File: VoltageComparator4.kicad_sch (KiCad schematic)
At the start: 6 parts, among them U18 LM324, U19 74LS08

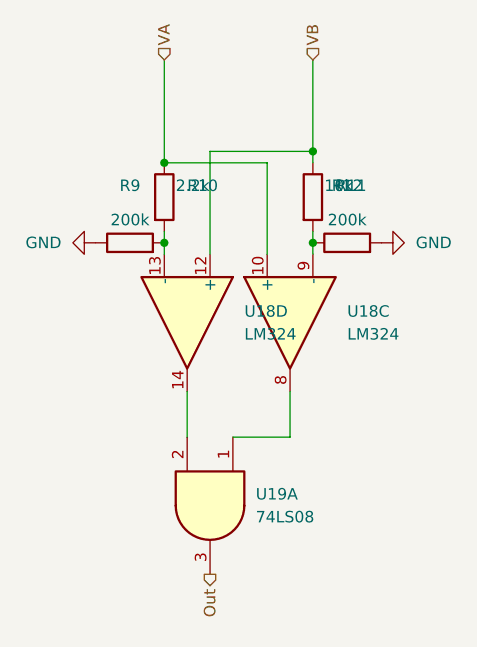
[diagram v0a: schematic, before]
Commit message: Ground and Power Plane?
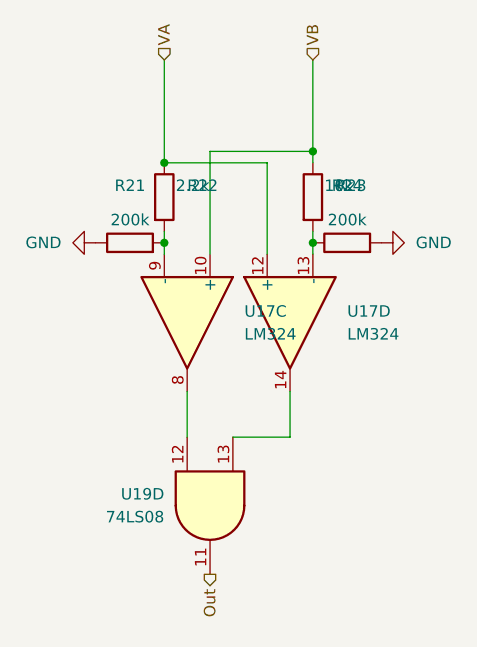
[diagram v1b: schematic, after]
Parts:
- renumbered R9 to R21, R10 to R22, R11 to R23, R12 to R24, U18 to U17
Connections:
- net Out: now also U19.11; no longer U19.3
- net VA: now also U17.12 (+); no longer U17.10 (+)
- net VB: now also U17.10 (+); no longer U17.12 (+)
- net at R21.2, R22.2: now also U17.9 (-); no longer U17.13 (-)
- net at R23.2, R24.1: now also U17.13 (-); no longer U17.9 (-)
- new net: U17.8, U19.12
- new net: U17.14, U19.13
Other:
- moved on the sheet: U19D
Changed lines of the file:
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@@
 	(symbol
 		(lib_id "74xx:74LS08")
-		(at 53.34 96.52 270)
-		(unit 1)
+		(at 53.34 96.52 90)
+		(mirror x)
+		(unit 4)
 		(exclude_from_sim no)
 		(in_bom yes)
@@
 		(dnp no)
 		(property "Reference" "U19"
-			(at 58.42 95.2416 90)
+			(at 48.26 95.2416 90)
 			(effects
 				(font
@@
 		)
 		(property "Value" "74LS08"
-			(at 58.42 97.7816 90)
+			(at 48.26 97.7816 90)
 			(effects
 				(font
@@
 		(dnp no)
 		(fields_autoplaced yes)
-		(property "Reference" "#PWR088"
+		(property "Reference" "#PWR094"
 			(at 78.74 67.31 0)
 			(effects
@@
 		(instances
 			(project "ECE145Mastermind"
-				(path "/8c64fe8a-5d6b-41bc-b3a3-9bda7b2e0f2c/4f59e726-7fd4-4ef0-8dbb-7a41976aa953"
-					(reference "#PWR088")
+				(path "/8c64fe8a-5d6b-41bc-b3a3-9bda7b2e0f2c/d4674d5d-47f2-4c8d-9fae-4e866cda3652"
+					(reference "#PWR094")
 					(unit 1)
 				)
@@
 		(on_board yes)
 		(dnp no)
-		(property "Reference" "R10"
+		(property "Reference" "R22"
 			(at 50.8 60.9599 0)
 			(effects
@@
 		(instances
 			(project "ECE145Mastermind"
-				(path "/8c64fe8a-5d6b-41bc-b3a3-9bda7b2e0f2c/4f59e726-7fd4-4ef0-8dbb-7a41976aa953"
-					(reference "R10")
+				(path "/8c64fe8a-5d6b-41bc-b3a3-9bda7b2e0f2c/d4674d5d-47f2-4c8d-9fae-4e866cda3652"
+					(reference "R22")
 					(unit 1)
 				)
@@
 		(dnp no)
 		(fields_autoplaced yes)
-		(property "Reference" "#PWR087"
+		(property "Reference" "#PWR093"
 			(at 34.29 67.31 0)
 			(effects
@@
 		(instances
 			(project "ECE145Mastermind"
-				(path "/8c64fe8a-5d6b-41bc-b3a3-9bda7b2e0f2c/4f59e726-7fd4-4ef0-8dbb-7a41976aa953"
-					(reference "#PWR087")
+				(path "/8c64fe8a-5d6b-41bc-b3a3-9bda7b2e0f2c/d4674d5d-47f2-4c8d-9fae-4e866cda3652"
+					(reference "#PWR093")
 					(unit 1)
 				)
@@
 		(on_board yes)
 		(dnp no)
-		(property "Reference" "R11"
+		(property "Reference" "R23"
 			(at 67.31 60.9599 0)
 			(effects
@@
 		(instances
 			(project "ECE145Mastermind"
-				(path "/8c64fe8a-5d6b-41bc-b3a3-9bda7b2e0f2c/4f59e726-7fd4-4ef0-8dbb-7a41976aa953"
-					(reference "R11")
+				(path "/8c64fe8a-5d6b-41bc-b3a3-9bda7b2e0f2c/d4674d5d-47f2-4c8d-9fae-4e866cda3652"
+					(reference "R23")
 					(unit 1)
 				)
@@
 		(at 62.23 76.2 90)
 		(mirror x)
-		(unit 3)
+		(unit 4)
 		(exclude_from_sim no)
 		(in_bom yes)
@@
 		(dnp no)
 		(fields_autoplaced yes)
-		(property "Reference" "U18"
+		(property "Reference" "U17"
 			(at 68.58 74.9299 90)
 			(effects
@@
 		(instances
 			(project "ECE145Mastermind"
-				(path "/8c64fe8a-5d6b-41bc-b3a3-9bda7b2e0f2c/4f59e726-7fd4-4ef0-8dbb-7a41976aa953"
-					(reference "U18")
-					(unit 3)
+				(path "/8c64fe8a-5d6b-41bc-b3a3-9bda7b2e0f2c/d4674d5d-47f2-4c8d-9fae-4e866cda3652"
+					(reference "U17")
+					(unit 4)
 				)
 			)
@@
 		(lib_id "Amplifier_Operational:LM324")
 		(at 50.8 76.2 270)
-		(unit 4)
+		(unit 3)
 		(exclude_from_sim no)
 		(in_bom yes)
@@
 		(dnp no)
 		(fields_autoplaced yes)
-		(property "Reference" "U18"
+		(property "Reference" "U17"
 			(at 57.15 74.9299 90)
 			(effects
@@
 		(instances
 			(project "ECE145Mastermind"
-				(path "/8c64fe8a-5d6b-41bc-b3a3-9bda7b2e0f2c/4f59e726-7fd4-4ef0-8dbb-7a41976aa953"
-					(reference "U18")
-					(unit 4)
+				(path "/8c64fe8a-5d6b-41bc-b3a3-9bda7b2e0f2c/d4674d5d-47f2-4c8d-9fae-4e866cda3652"
+					(reference "U17")
+					(unit 3)
 				)
 			)
@@
 		(on_board yes)
 		(dnp no)
-		(property "Reference" "R9"
+		(property "Reference" "R21"
 			(at 44.45 60.96 90)
 			(effects
@@
 		(instances
 			(project "ECE145Mastermind"
-				(path "/8c64fe8a-5d6b-41bc-b3a3-9bda7b2e0f2c/4f59e726-7fd4-4ef0-8dbb-7a41976aa953"
-					(reference "R9")
+				(path "/8c64fe8a-5d6b-41bc-b3a3-9bda7b2e0f2c/d4674d5d-47f2-4c8d-9fae-4e866cda3652"
+					(reference "R21")
 					(unit 1)
 				)
@@
 		(on_board yes)
 		(dnp no)
-		(property "Reference" "R12"
+		(property "Reference" "R24"
 			(at 68.58 60.96 90)
 			(effects
@@
 		(instances
 			(project "ECE145Mastermind"
-				(path "/8c64fe8a-5d6b-41bc-b3a3-9bda7b2e0f2c/4f59e726-7fd4-4ef0-8dbb-7a41976aa953"
-					(reference "R12")
+				(path "/8c64fe8a-5d6b-41bc-b3a3-9bda7b2e0f2c/d4674d5d-47f2-4c8d-9fae-4e866cda3652"
+					(reference "R24")
 					(unit 1)
 				)

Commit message: Finished?
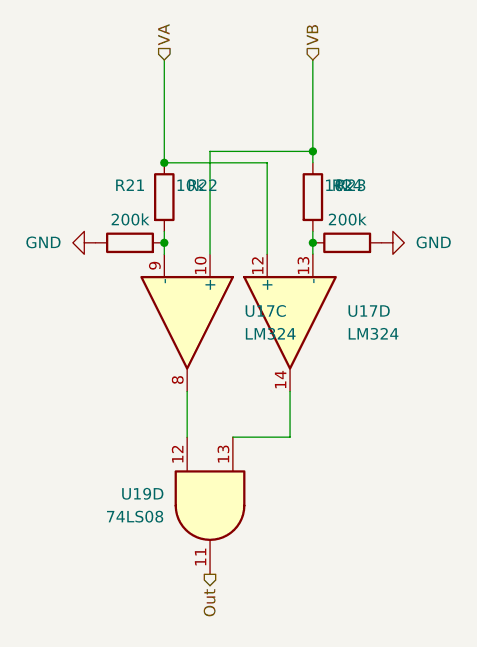
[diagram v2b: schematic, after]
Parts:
- R22: value 2.2k -> 10k
